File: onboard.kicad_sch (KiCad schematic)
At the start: 16 parts, among them Q2 2N7002K, Q3 2N7002, SW3 SW_DIP_x08, SW4 User, U6 SA39-11EWA, U7 SA39-11EWA

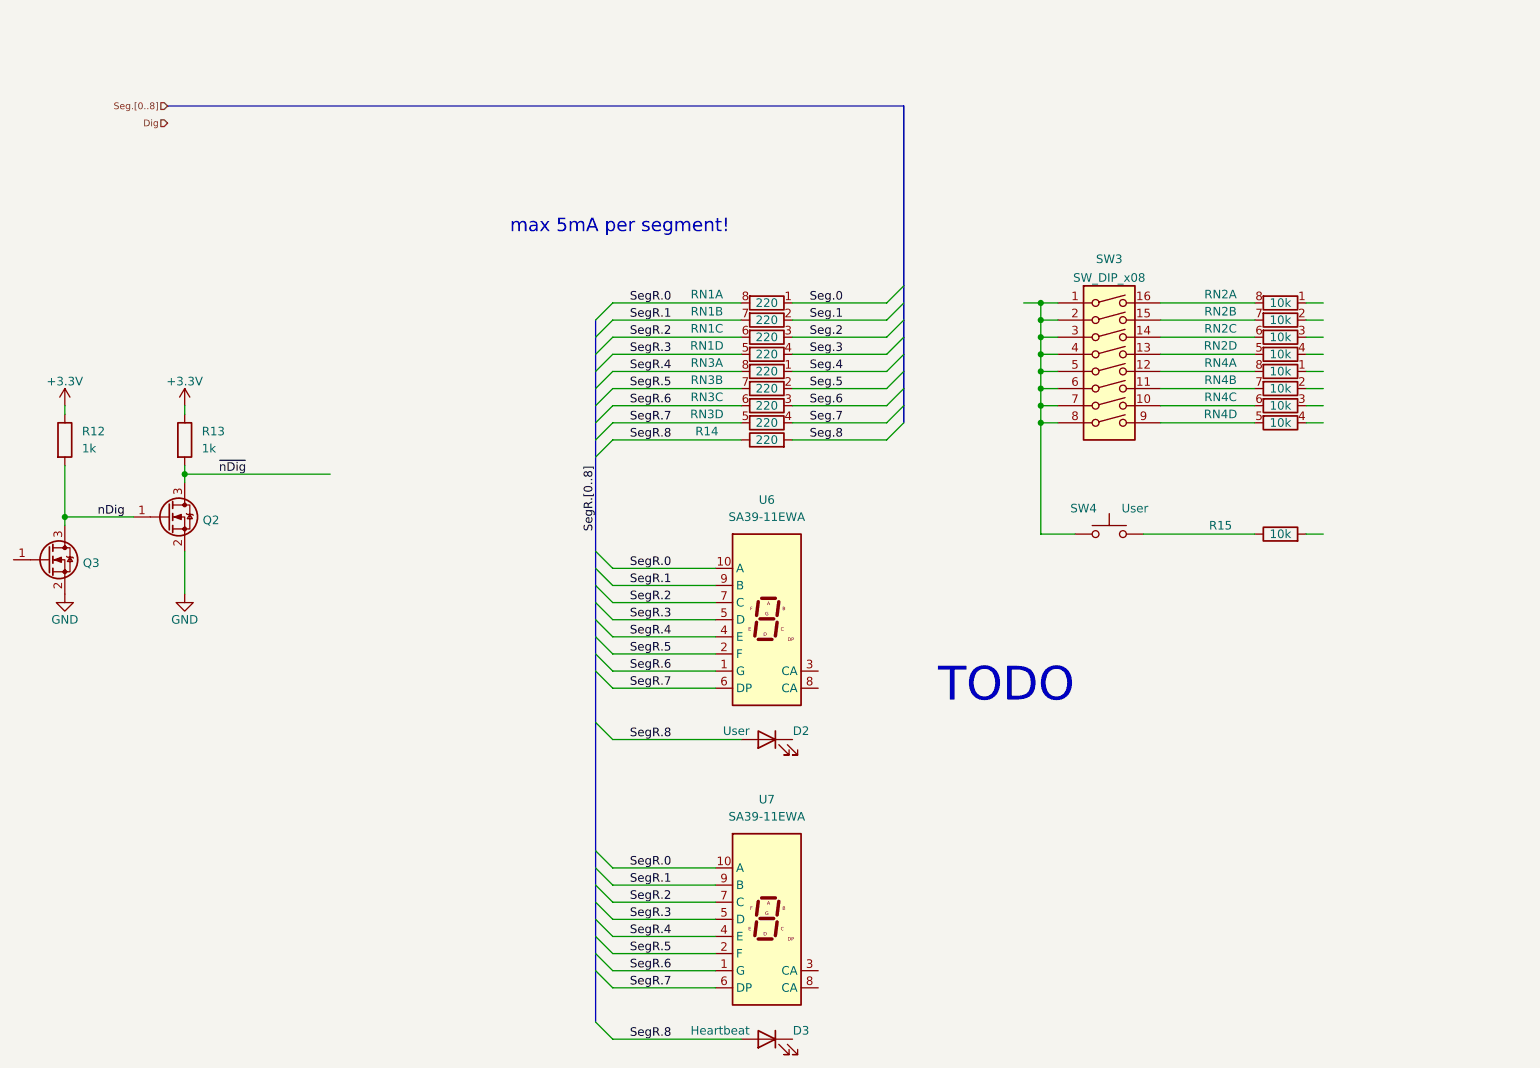
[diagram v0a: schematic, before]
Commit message: Done?
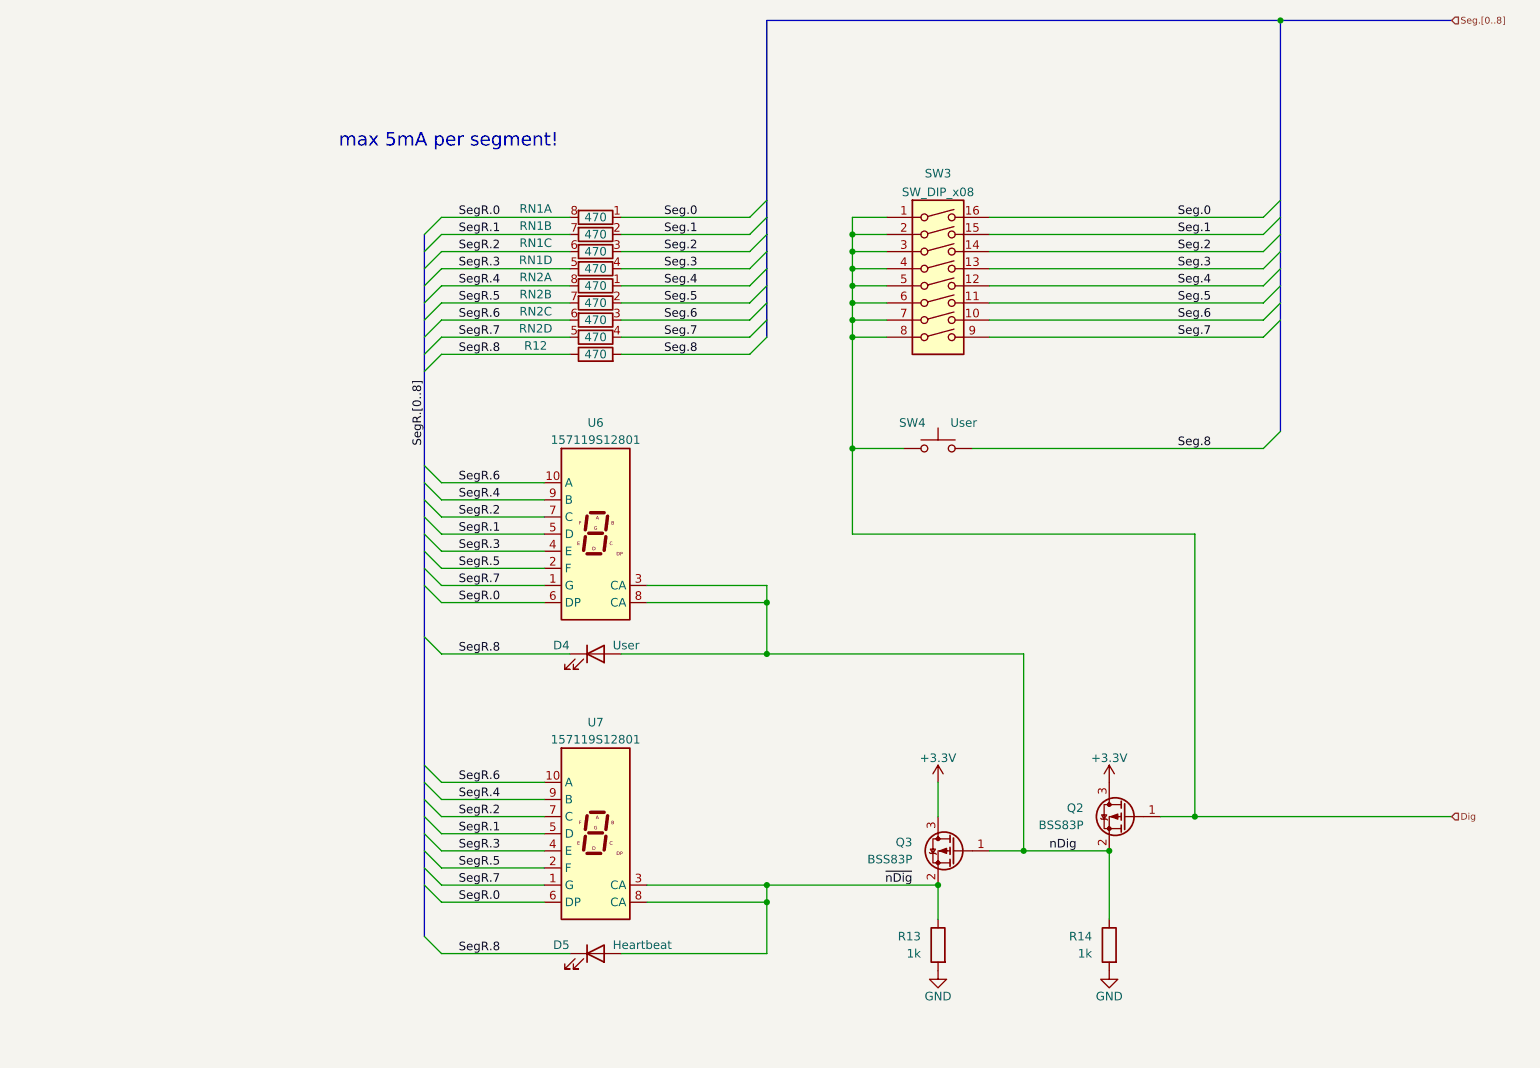
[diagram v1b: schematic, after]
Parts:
- removed Q2: 2N7002K, Package_TO_SOT_SMD:SOT-23, symbol Transistor_FET:2N7002K
- removed Q3: 2N7002, Package_TO_SOT_SMD:SOT-23, symbol Transistor_FET:2N7002
- removed R15: 10k, Resistor_SMD:R_0603_1608Metric, symbol Device:R
- removed RN2, RN4: 10k, Resistor_SMD:R_Array_Convex_4x0603, symbol Device:R_Pack04_Split
- added Q2, Q3: BSS83P, Package_TO_SOT_SMD:SOT-23, symbol Transistor_FET:BSS83P
- R12: renamed from R14; value 220 -> 470
- RN1: value 220 -> 470
- RN2: renamed from RN3; value 220 -> 470
- U6, U7: value SA39-11EWA -> 157119S12801
- renumbered D2 to D4, D3 to D5, R12 to R14
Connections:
- net +3V3: now also Q2.3 (D), Q3.3 (D); no longer R13.1, R14.1
- net Dig: now also SW3.1, SW3.2, SW3.3, SW3.4, SW3.5, SW3.6, SW3.7, SW3.8, SW4.1, Q2.1 (G)
- net GND: now also R13.2, R14.2
- net Seg.0: now also SW3.16
- net Seg.1: now also SW3.15
- net Seg.2: now also SW3.14
- net Seg.3: now also SW3.13
- net Seg.4: now also SW3.12
- net Seg.5: now also SW3.11
- net Seg.6: now also SW3.10
- net Seg.7: now also SW3.9
- net Seg.8: now also SW4.2
- net SegR.0: now also U6.6 (DP), U7.6 (DP); no longer U6.10 (A), U7.10 (A)
- net SegR.1: now also U6.5 (D), U7.5 (D); no longer U6.9 (B), U7.9 (B)
- net SegR.3: now also U6.4 (E), U7.4 (E); no longer U6.5 (D), U7.5 (D)
- net SegR.4: now also U6.9 (B), U7.9 (B); no longer U6.4 (E), U7.4 (E)
- net SegR.6: now also U6.10 (A), U7.10 (A); no longer U6.1 (G), U7.1 (G)
- net SegR.7: now also U6.1 (G), U7.1 (G); no longer U6.6 (DP), U7.6 (DP)
- net SegR.8: now also D4.1 (K), D5.1 (K); no longer D4.2 (A), D5.2 (A)
- net nDig: now also D4.2 (A), R14.1, U6.3 (CA), U6.8 (CA), Q2.2 (S), Q3.1 (G); no longer R14.2
- net ~{nDig}: now also D5.2 (A), R13.1, U7.3 (CA), U7.8 (CA), Q3.2 (S); no longer R13.2
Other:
- note removed: "TODO"
- moved on the sheet: D4, D5, R12, R13, R14, RN1A, RN1B, RN1C, RN1D, RN2A, RN2B, RN2C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
